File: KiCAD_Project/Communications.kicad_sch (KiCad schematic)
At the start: 23 parts, among them J14 1-0000050, J15 1-0000190, U10 1-0000785, U12 1-0000464

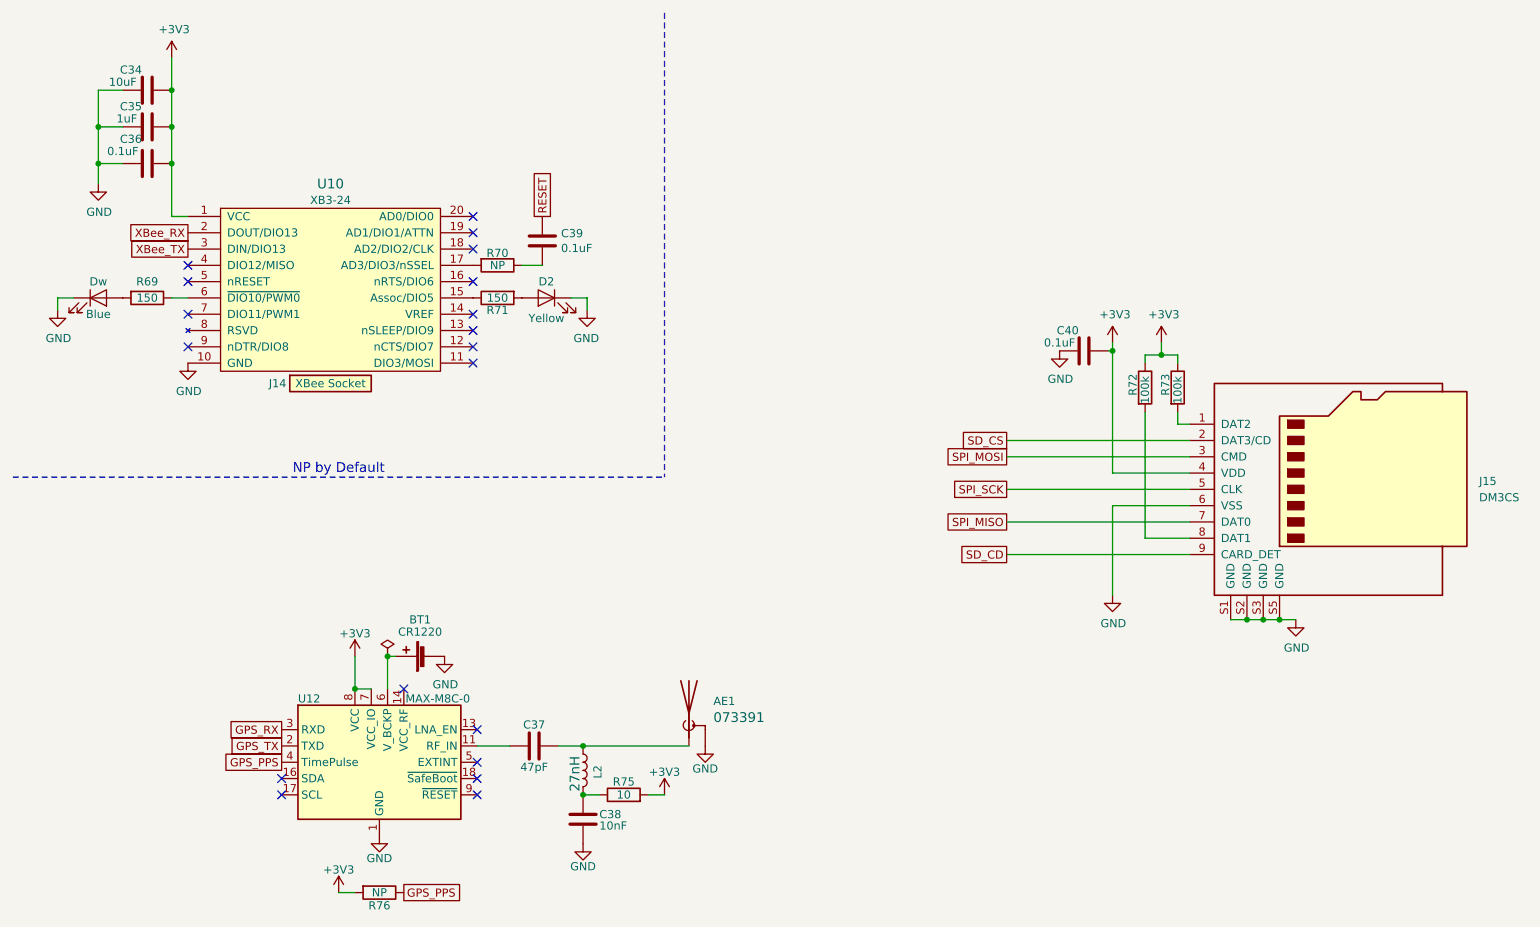
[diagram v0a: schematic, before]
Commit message: Schematic ERC Issue Cleanup
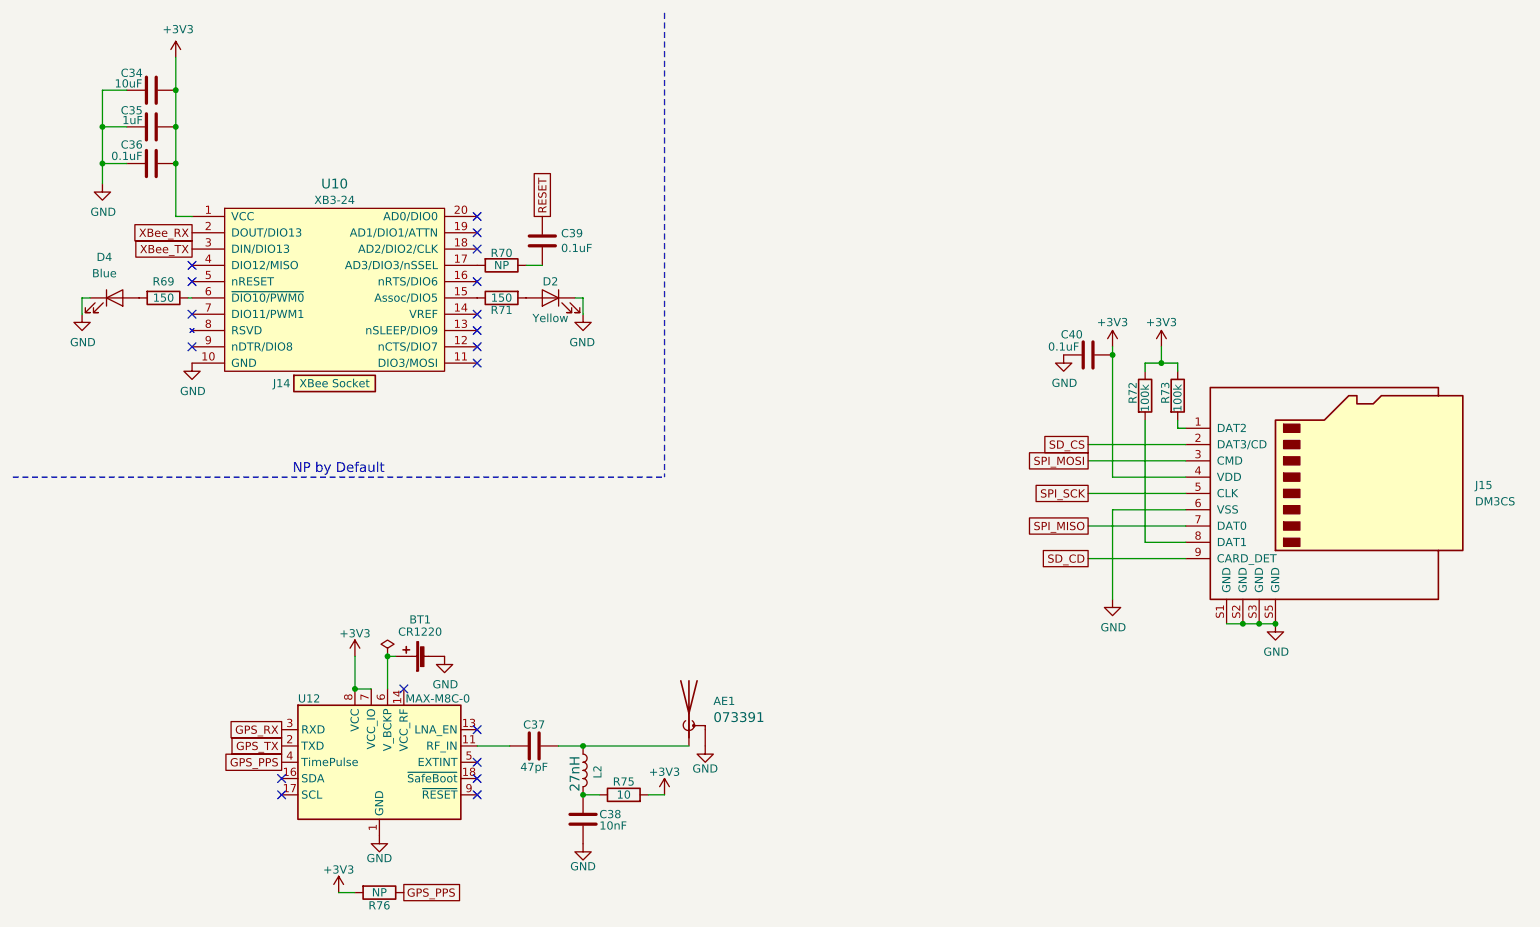
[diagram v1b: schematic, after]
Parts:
- removed Dw: 1-0000599, leds_0805:1-0000599, symbol leds_0805:1-0000599
- added D4: 1-0000599, leds_0805:1-0000599, symbol leds_0805:1-0000599
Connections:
- net GND: now also D4.1 (K)
- net at R69.2: now also D4.2 (A)
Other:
- moved on the sheet: C34, C35, C36, C40, D2, J14, J15, R69, R70, R71, R72, R73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
